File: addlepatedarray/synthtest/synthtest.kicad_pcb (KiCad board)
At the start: 2 copper layers, 65 x 30 mm, 72 parts, among them J1 RF0A+, J2 RF0A-, J3 RF0B-, J4 RF0B+, J5 RF1A-, J6 RF1B-, J7 RF1A+, J8 RF1B+, J9 REF, U1 ADF4351, U2 ADF4351, U4 CH32V003FxUx, U6 LDL1117-33, Y1 TG-5006CG-12H 26.0000M3

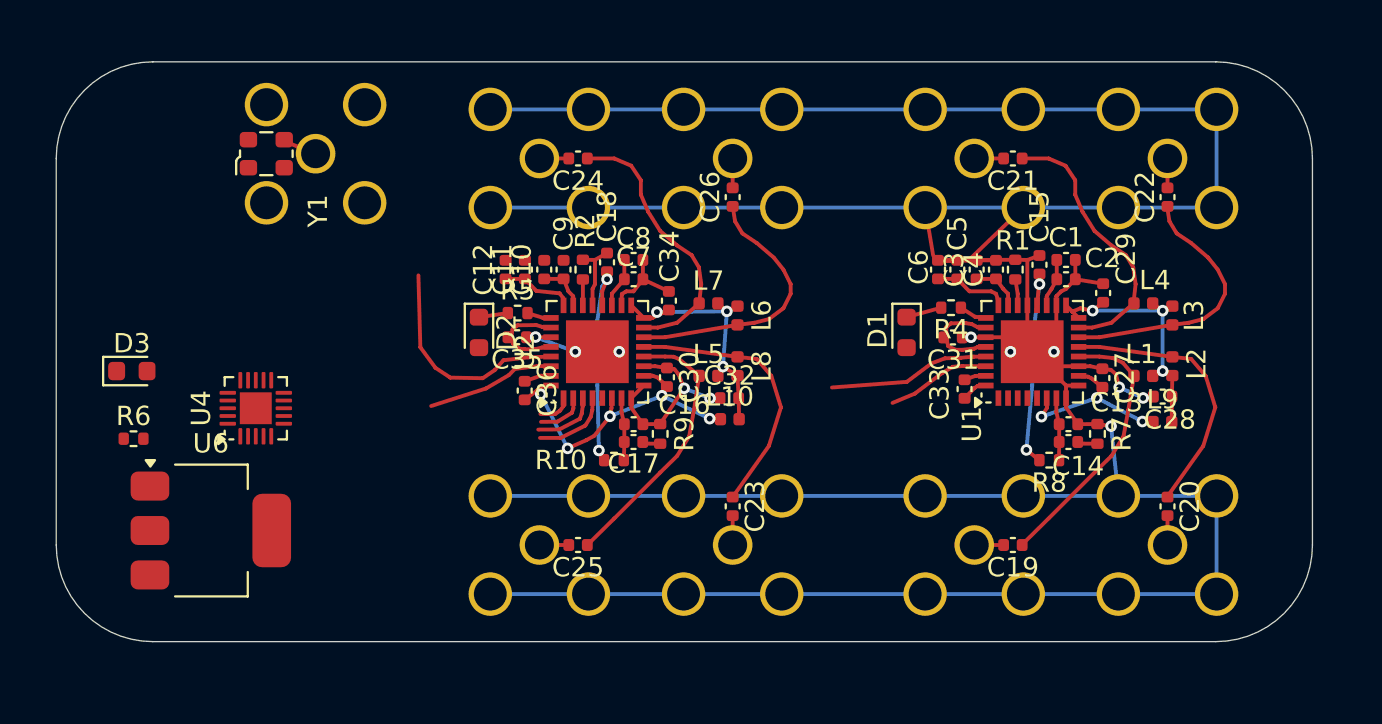
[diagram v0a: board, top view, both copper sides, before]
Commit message: Bump disign!
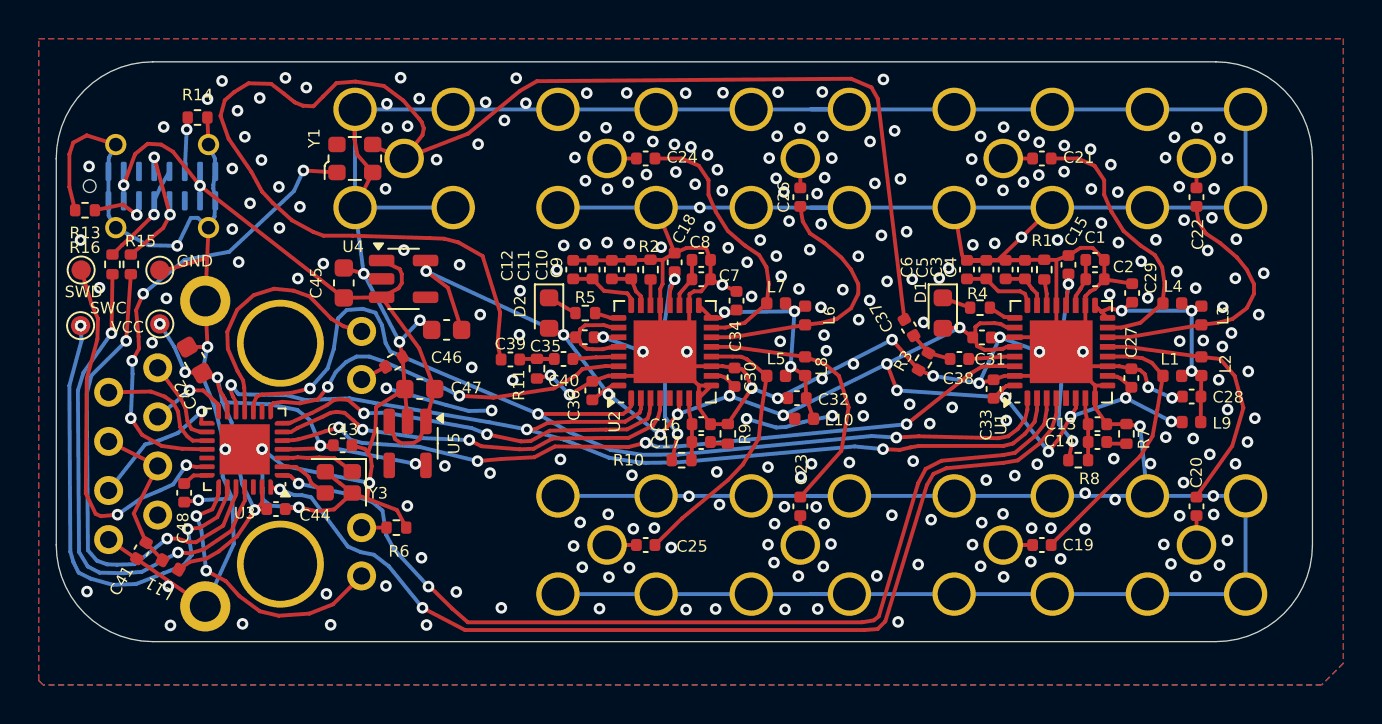
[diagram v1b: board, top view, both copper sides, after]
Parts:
- removed D3: LEDPWR, LED_SMD:LED_0603_1608Metric
- removed U6: LDL1117-33, Package_TO_SOT_SMD:SOT-223-3_TabPin2
- added C37: 1n, Capacitor_SMD:C_0402_1005Metric, F.Cu at (189.1, 38.8)
- added C38: 1n, Capacitor_SMD:C_0402_1005Metric, F.Cu at (191.7, 40.4)
- added C39: 1n, Capacitor_SMD:C_0402_1005Metric, F.Cu at (168.5, 40.4)
- added C40: 1n, Capacitor_SMD:C_0402_1005Metric, F.Cu at (171.2, 40.4)
- added C41: 1u, Capacitor_SMD:C_0402_1005Metric, F.Cu at (149.4, 50.3)
- added C42: 4.7u, Capacitor_SMD:C_0603_1608Metric, F.Cu at (152.2, 40.4)
- added C43: 1u, Capacitor_SMD:C_0402_1005Metric, F.Cu at (159.8, 44.8)
- added C44: 1u, Capacitor_SMD:C_0402_1005Metric, F.Cu at (156.4, 48.1)
- added C45: 4.7u, Capacitor_SMD:C_0603_1608Metric, F.Cu at (159.9, 36.4)
- added C46: 4.7u, Capacitor_SMD:C_0603_1608Metric, F.Cu at (165.2, 38.9)
- added C47: 4.7u, Capacitor_SMD:C_0603_1608Metric, F.Cu at (163.8, 41.9)
- added C48: 1u, Capacitor_SMD:C_0402_1005Metric, F.Cu at (151.6, 47.3)
- added J10: RJ45_Hanrun_HR911105A_Horizontal, cnhardware:HR915310A-RJ45-INTEGRATED-10MBIT, B.Cu at (156.6, 45.3)
- added J11: USB_C_Receptacle_USB2.0_14P, Connector_USB:USB_C_Receptacle_G-Switch_GT-USB-7051x, B.Cu at (150.5, 31.4)
- added J12: VCC, TestPoint:TestPoint_Pad_D1.0mm, F.Cu at (150.4, 38.6)
- added J13: SWC, TestPoint:TestPoint_Pad_D1.0mm, F.Cu at (146.3, 38.6)
- added J14: SWD, TestPoint:TestPoint_Pad_D1.0mm, F.Cu at (146.3, 35.8)
- added J15: GND, TestPoint:TestPoint_Pad_D1.0mm, F.Cu at (150.4, 35.8)
- added L11: 3.9nH, Inductor_SMD:L_0402_1005Metric, F.Cu at (150.9, 51.0)
- added R11: 100, Resistor_SMD:R_0402_1005Metric, F.Cu at (169.9, 40.9)
- added R12: 1.5k, cnhardware:R_0402_1005Metric_COMPACT, F.Cu at (162.5, 40.5)
- added R13: 5.1k, Resistor_SMD:R_0402_1005Metric, F.Cu at (146.5, 32.7)
- added R14: 5.1k, Resistor_SMD:R_0402_1005Metric, F.Cu at (152.3, 27.9)
- added R15: 33, Resistor_SMD:R_0402_1005Metric, F.Cu at (148.9, 35.5)
- added R16: 33, Resistor_SMD:R_0402_1005Metric, F.Cu at (147.9, 35.5)
- added R3: 100, Resistor_SMD:R_0402_1005Metric, F.Cu at (189.9, 40.5)
- added U3: CH32V208GBU6, Package_DFN_QFN:QFN-28-1EP_4x4mm_P0.45mm_EP2.6x2.6mm, F.Cu at (154.8, 45.0)
- added U5: WL2808E, Package_TO_SOT_SMD:SOT-23-5, F.Cu at (163.2, 44.7)
- added Y3: 32MHz, Crystal:Crystal_SMD_2016-4Pin_2.0x1.6mm, F.Cu at (159.6, 46.8)
- U4: value CH32V003FxUx -> WL2808E; footprint Package_DFN_QFN:QFN-20-1EP_3x3mm_P0.4mm_EP1.65x1.65mm -> Package_TO_SOT_SMD:SOT-23-5
- moved R6 14.4 mm to (162.6, 49.1)
- moved U4 10.2 mm to (163.0, 36.2), turned to 0 degrees
- moved J9 4.59 mm to (163.0, 30.0)
- moved Y1 4.59 mm to (160.5, 30.0)
- moved L10 3.85 mm to (183.7, 43.5)
- moved D2 3.76 mm to (170.5, 38.0)
- moved C10 3.50 mm to (173.8, 35.8)
- moved C11 3.50 mm to (172.8, 35.8)
- moved C12 3.50 mm to (171.8, 35.8)
- moved C16 3.50 mm to (178.4, 43.8)
- moved C17 3.50 mm to (178.4, 44.7)
- moved C18 3.50 mm to (177.0, 35.4)
- moved C23 3.50 mm to (183.5, 48.0)
- moved C24 3.50 mm to (175.5, 30.0)
- moved C25 3.50 mm to (175.5, 50.0)
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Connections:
- U1 pad 29: REFCLK -> Net-(U1-REFIN)
- U2 pad 29: REFCLK -> Net-(U2-REFIN)
- U4 pad 1: CE1 -> +5V
- U4 pad 2: unconnected-(U4-PA1-Pad2) -> GND
- U4 pad 3: unconnected-(U4-PA2-Pad3) -> +5V
- U4 pad 4: GND -> unconnected-(U4-NC-Pad4)
- U4 pad 5: unconnected-(U4-PD0-Pad5) -> +3.3V
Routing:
- net GND: track 235.9 -> 423.0 mm, vias 11 -> 283
- net REFCLK: track 21.8 -> 77.2 mm
- net CE0: track 0.00 -> 51.4 mm, vias 0 -> 2
- net SCK: track 1.78 -> 52.9 mm, vias 0 -> 3
- net LE0: track 0.00 -> 50.8 mm, vias 0 -> 2
- net MOSI: track 2.50 -> 52.3 mm, vias 0 -> 3
- net +3.3V: track 37.7 -> 79.2 mm, vias 8 -> 15
- net +3V3: track 0.00 -> 36.6 mm, vias 0 -> 6
- net MUXOUT0: track 5.37 -> 39.7 mm, vias 0 -> 4
- net +5V: track 0.00 -> 33.6 mm, vias 0 -> 2
- net D+: track 0.00 -> 26.3 mm, vias 0 -> 2
- net D-: track 0.00 -> 25.2 mm, vias 0 -> 2
- net SWC: track 0.00 -> 24.1 mm, vias 0 -> 2
- net XTALEN: track 0.00 -> 23.8 mm, vias 0 -> 4
- net SWD: track 0.00 -> 19.7 mm, vias 0 -> 2
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- added copper zone on B.Cu, net GND
- added copper zone on F.Cu, net GND
